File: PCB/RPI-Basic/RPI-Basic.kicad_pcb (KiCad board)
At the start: 2 copper layers, 90 x 90 mm, 2 parts, among them J1 SE2-30, J2 Conn_02x20_Odd_Even

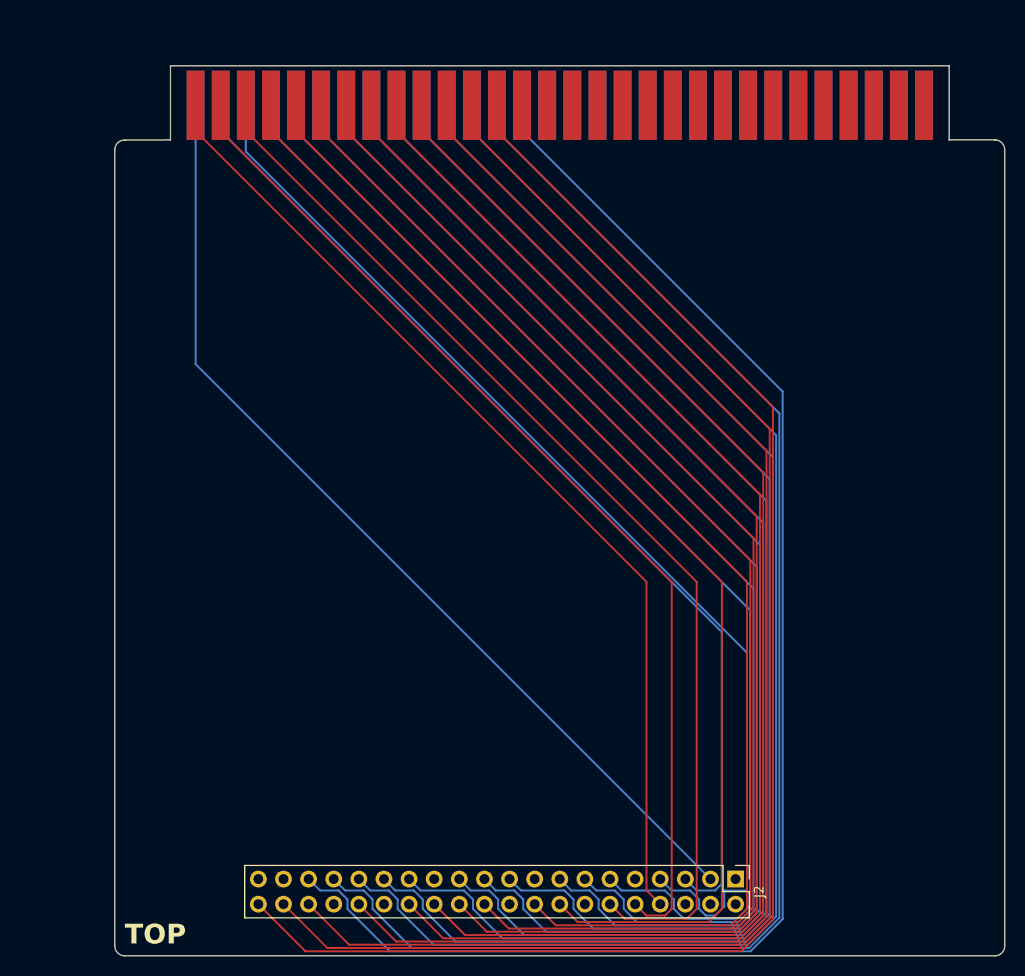
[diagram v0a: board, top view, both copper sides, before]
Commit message: layed out board
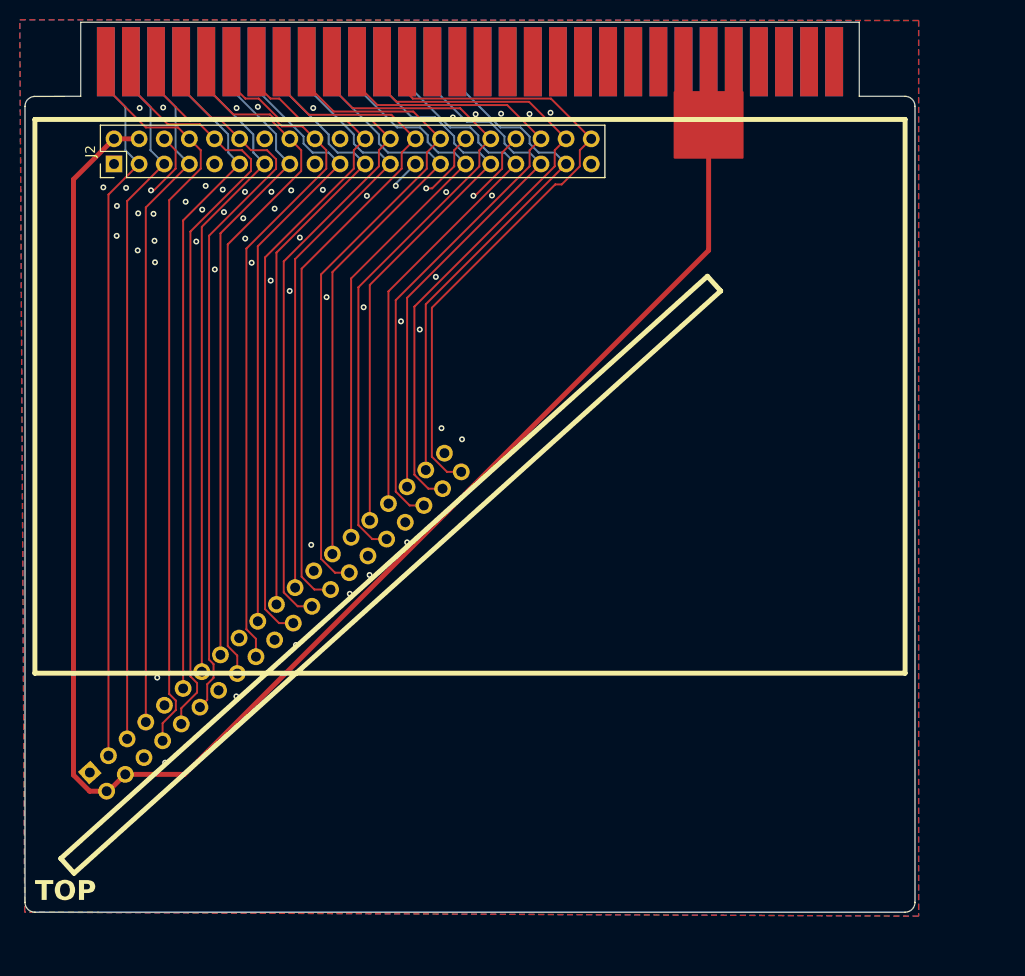
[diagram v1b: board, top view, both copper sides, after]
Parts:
- added J3: Conn_02x20_Odd_Even, Connector_PinHeader_2.54mm:PinHeader_2x20_P2.54mm_Vertical, B.Cu at (103.4, 120.0)
- moved J2 95.8 mm to (105.9, 58.5), turned to 90 degrees
- moved J1 10.1 mm to (141.9, 48.1)
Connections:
- J1 pad 23: +3.3V -> unconnected-(J1-3.3V-Pad23)
- J1 pad 53: +3.3V -> unconnected-(J1-3.3V-Pad53)
- J2 pad 1: +3.3V -> unconnected-(J2-Pin_1-Pad1)
- J2 pad 17: +3.3V -> unconnected-(J2-Pin_17-Pad17)
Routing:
- net +5V: track 0.00 -> 171.4 mm
- net /19: track 146.1 -> 55.5 mm
- net /13: track 143.8 -> 56.7 mm
- net /6: track 141.5 -> 58.3 mm
- net /21: track 149.2 -> 66.5 mm
- net /20: track 146.9 -> 67.1 mm
- net /5: track 139.2 -> 59.8 mm
- net /16: track 144.6 -> 68.4 mm
- net /0: track 136.9 -> 61.3 mm
- net /12: track 139.8 -> 68.9 mm
- net /11: track 132.0 -> 61.6 mm
- net /9: track 129.7 -> 63.1 mm
- net /1: track 134.9 -> 69.0 mm
- net /10: track 127.4 -> 64.5 mm
- net /7: track 132.6 -> 70.8 mm
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- added copper zone on B.Cu, net GND
- added copper zone on F.Cu, net GND
